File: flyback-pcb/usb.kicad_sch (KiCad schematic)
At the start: 0 parts

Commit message: USB+protection
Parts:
- added C1, C2, C5: C, Capacitor_SMD:C_0603_1608Metric, symbol Device:C
- added D1: 824012823, emc_flyback_pcb:WE-TVS_DFN1210-6L, symbol emc_flyback_pcb:824012823
- added D2: 824045810, emc_flyback_pcb:WE-TVS_DFN1610-2L, symbol emc_flyback_pcb:824045810
- added J1: MUSBRM1C130, MUSBRM1C130:AMPHENOL_MUSBRM1C130, symbol 34654_flyback_pcb:MUSBRM1C130
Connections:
- new net: C1.2, J1.A4
- new net CC1: C2.2, D1.1 (K1), J1.A5
- new net CC2: C5.1, D1.2 (K2), J1.B5
- new net DPI+: J1.A6, J1.B6
- new net DPI-: J1.A7, J1.B7
- new net GND: C1.1, C2.1, C5.2, D1.3 (A), D2.2 (A2), J1.A1, J1.A12, J1.B1, J1.B12, J1.G1 (GND), J1.G2 (GND), J1.G3 (GND), J1.G4 (GND), J1.G5 (GND), J1.G6 (GND), J1.S1 (SHIELD), J1.S2 (SHIELD)
- new net VBUS: D2.1 (A1)
- no-connect marks 0 -> 10

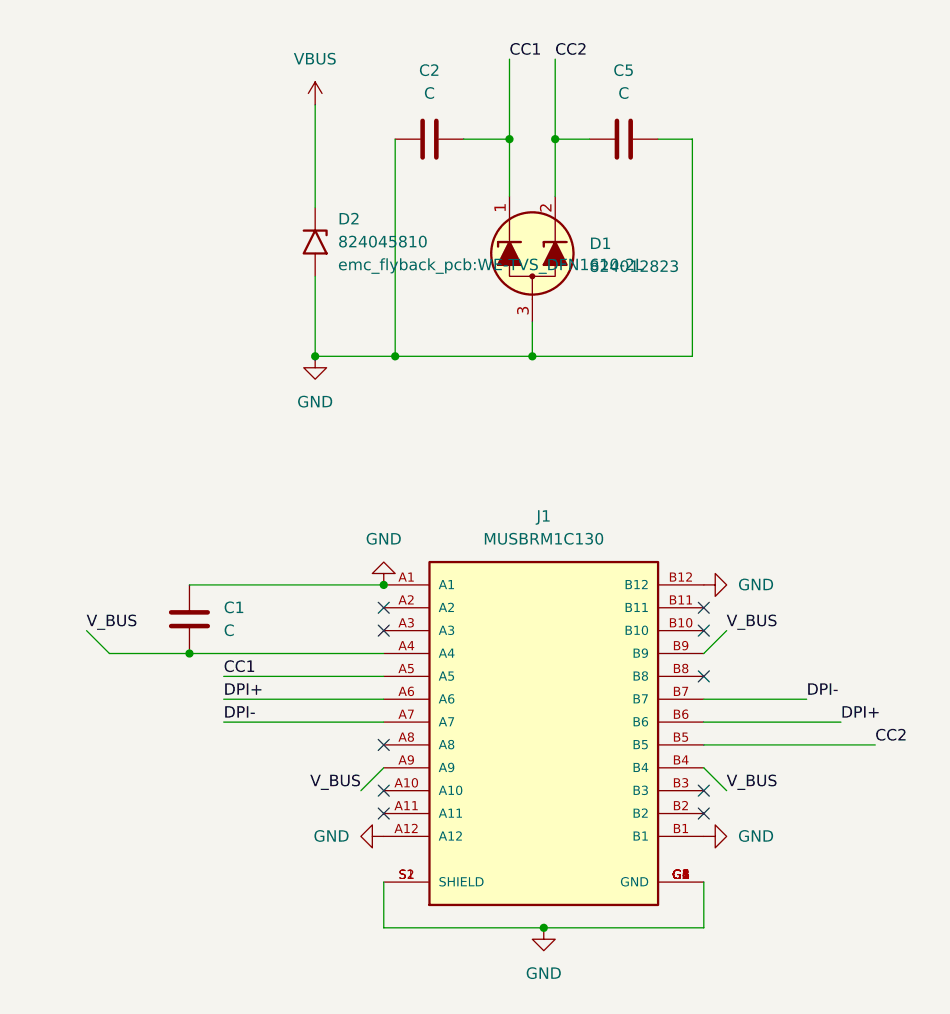
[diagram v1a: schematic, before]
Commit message: Re-done USB
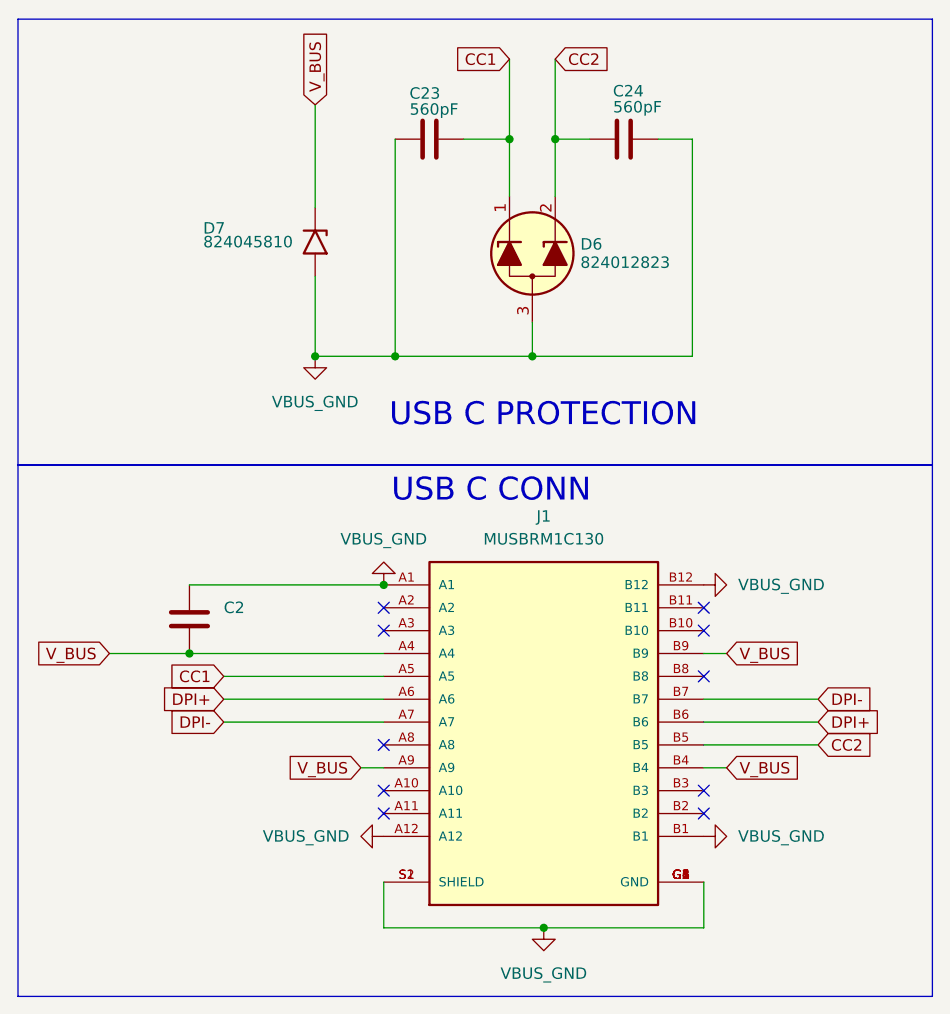
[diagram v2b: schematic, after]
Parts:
- C23: renamed from C2; value C -> 560pF
- C24: renamed from C5; value C -> 560pF
- renumbered C1 to C2, D1 to D6, D2 to D7
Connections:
- net VBUS is gone; now on net V_BUS: D7.1 (A1)
- net V_BUS: now also C2.2, J1.A4, J1.A9, J1.B4, J1.B9
- net GND renamed VBUS_GND
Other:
- note added: "USB C CONN"
- note added: "USB C PROTECTION"
